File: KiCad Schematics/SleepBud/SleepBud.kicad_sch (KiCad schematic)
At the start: 6 parts, among them U1 ESP32-S3-WROOM-1, U2 DS3231SN_, U3 AM312, U4 AMS1117-3.3, U5 AMS1117-5.0

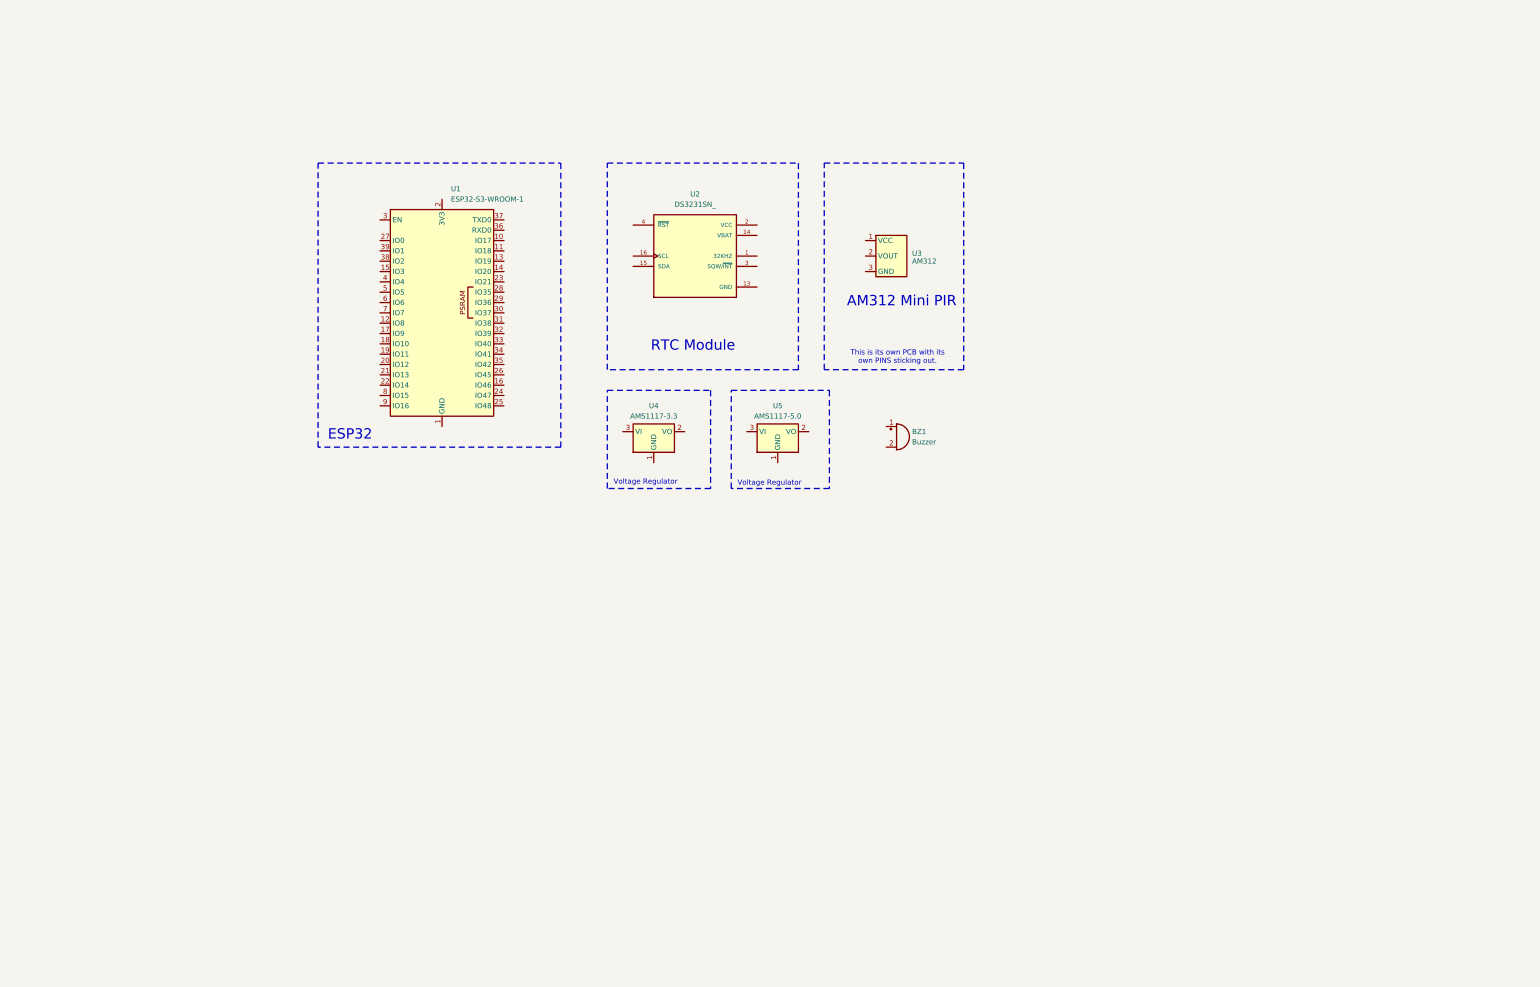
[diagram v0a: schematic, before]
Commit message: Version 10/25
Added connections
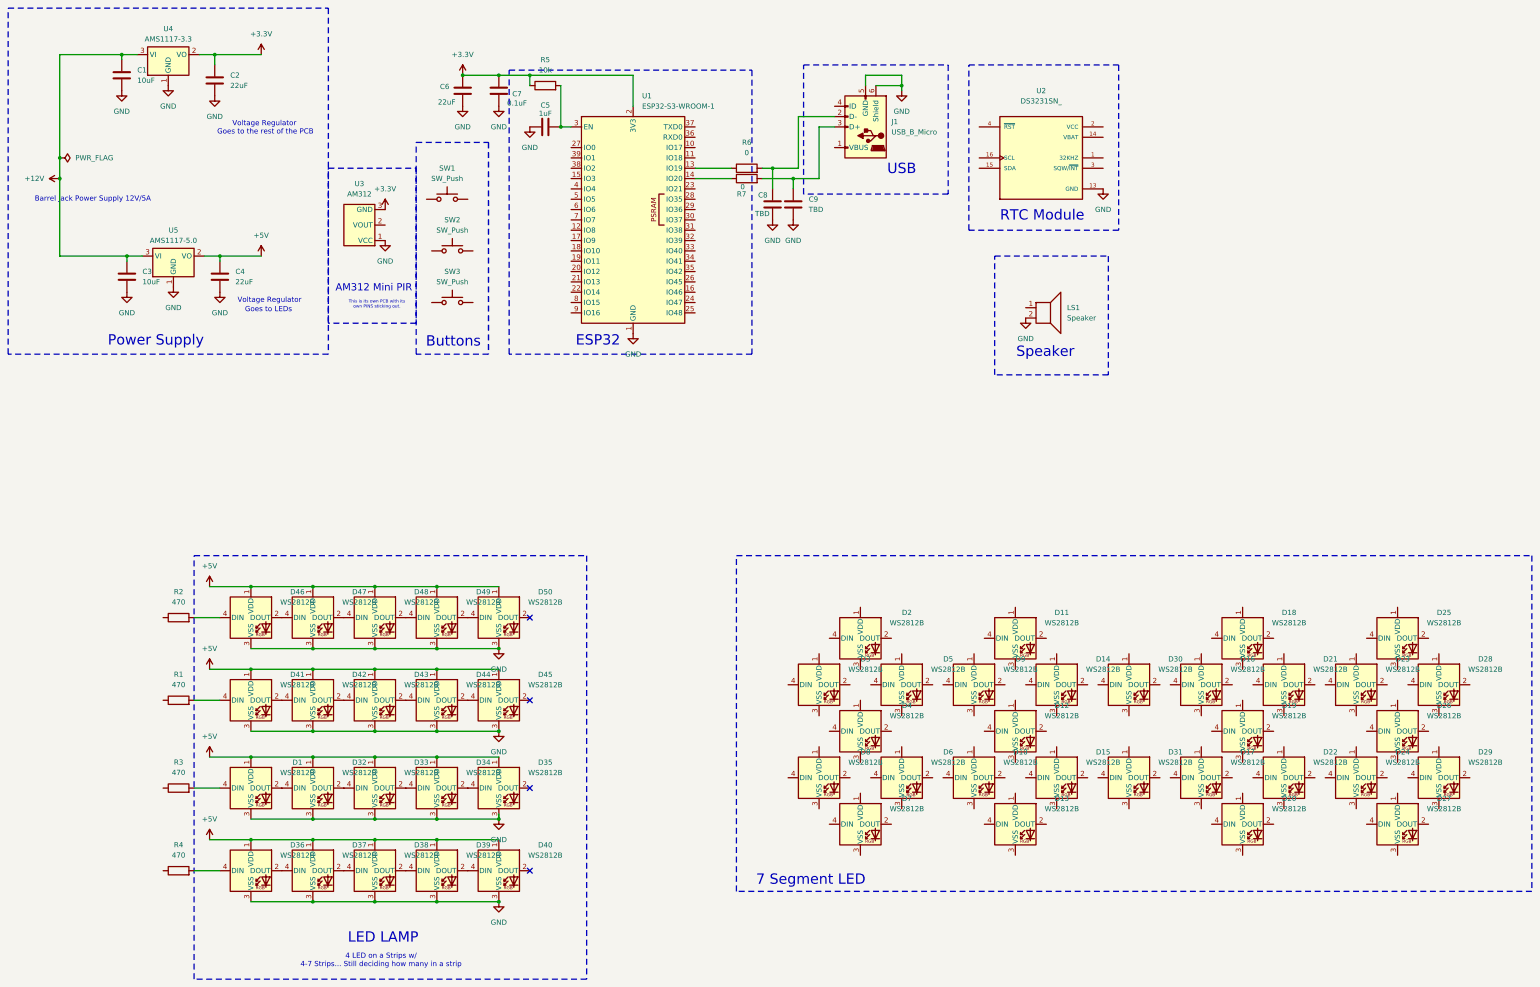
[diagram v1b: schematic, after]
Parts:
- removed BZ1: Buzzer, symbol Device:Buzzer
- added C1, C3: 10uF, symbol Device:C
- added C2, C4, C6: 22uF, symbol Device:C
- added C5: 1uF, symbol Device:C
- added C7: 0.1uF, symbol Device:C
- added C8, C9: TBD, symbol Device:C
- added D1, D10, D11, D12, D13, D14, D15, D16, D17, D18, D19, D2, D20, D21, D22, D23, D24, D25, D26, D27, D28, D29, D3, D30, D31, D32, D33, D34, D35, D36, D37, D38, D39, D4, D40, D41, D42, D43, D44, D45, D46, D47, D48, D49, D5, D50, D6, D7, D8, D9: WS2812B, LED_SMD:LED_WS2812B_PLCC4_5.0x5.0mm_P3.2mm, symbol LED:WS2812B
- added J1: USB_B_Micro, symbol Connector:USB_B_Micro
- added LS1: Speaker, symbol Device:Speaker
- added R1, R2, R3, R4: 470, symbol Device:R
- added R5: 10k, symbol Device:R
- added R6, R7: 0, symbol Device:R
- added SW1, SW2, SW3: SW_Push, symbol Switch:SW_Push
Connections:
- net GND: now reaches U2.13 (GND)
- net GND: now also U1.1 (GND), U1.40 (GND), U1.41 (GND), U3.1 (VCC), U4.1 (GND), U5.1 (GND), C1.2, C2.2, C3.2, C4.2, C5.1, C6.2, C7.2, C8.2, C9.2, D1.3 (VSS), D32.3 (VSS), D33.3 (VSS), D34.3 (VSS), D35.3 (VSS), D36.3 (VSS), D37.3 (VSS), D38.3 (VSS), D39.3 (VSS), D40.3 (VSS), D41.3 (VSS), D42.3 (VSS), D43.3 (VSS), D44.3 (VSS), D45.3 (VSS), D46.3 (VSS), D47.3 (VSS), D48.3 (VSS), D49.3 (VSS), D50.3 (VSS), J1.5 (GND), J1.6 (Shield), LS1.2
- net +5V: now reaches U5.2 (VO)
- net +5V: now also C4.1, D1.1 (VDD), D32.1 (VDD), D33.1 (VDD), D34.1 (VDD), D35.1 (VDD), D36.1 (VDD), D37.1 (VDD), D38.1 (VDD), D39.1 (VDD), D40.1 (VDD), D41.1 (VDD), D42.1 (VDD), D43.1 (VDD), D44.1 (VDD), D45.1 (VDD), D46.1 (VDD), D47.1 (VDD), D48.1 (VDD), D49.1 (VDD), D50.1 (VDD)
- net +12V: now reaches U5.3 (VI)
- net +12V: now also U4.3 (VI), C1.1, C3.1
- net at U1.13 (IO19): now also R6.1
- net at U1.14 (IO20): now also R7.1
- net +3.3V: now reaches U1.2 (3V3)
- net +3.3V: now also U3.3 (GND), U4.2 (VO), C2.1, C6.1, C7.1, R5.1
- net at U1.3 (EN): now also C5.2, R5.2
- new net: D37.2 (DOUT), D38.4 (DIN)
- new net: D36.2 (DOUT), D37.4 (DIN)
- new net: D44.2 (DOUT), D45.4 (DIN)
- new net: D43.2 (DOUT), D44.4 (DIN)
- new net: D1.4 (DIN), R3.2
- new net: D41.4 (DIN), R1.2
- new net: D1.2 (DOUT), D32.4 (DIN)
- new net: D39.2 (DOUT), D40.4 (DIN)
- new net: D38.2 (DOUT), D39.4 (DIN)
- new net: D33.2 (DOUT), D34.4 (DIN)
- new net: D32.2 (DOUT), D33.4 (DIN)
- new net: D47.2 (DOUT), D48.4 (DIN)
- new net: D46.2 (DOUT), D47.4 (DIN)
- new net: C9.1, J1.3 (D+), R7.2
- new net: D42.2 (DOUT), D43.4 (DIN)
- new net: D41.2 (DOUT), D42.4 (DIN)
- new net: D49.2 (DOUT), D50.4 (DIN)
- new net: D48.2 (DOUT), D49.4 (DIN)
- new net: D34.2 (DOUT), D35.4 (DIN)
- new net: D46.4 (DIN), R2.2
- new net: D36.4 (DIN), R4.2
- new net: C8.1, J1.2 (D-), R6.2
- no-connect marks 0 -> 4
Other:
- note added: "4 LED on a Strips w/ 4-7 Strips... Still deciding how many in a strip"
- note added: "7 Segment LED"
- note added: "Barrel Jack Power Supply 12V/5A"
- note added: "Buttons"
- note added: "Goes to LEDs"
- note added: "Goes to the rest of the PCB"
- note added: "LED LAMP"
- note added: "Power Supply"
- note added: "Speaker"
- note added: "USB"
- moved on the sheet: U1, U2, U3, U4, U5
